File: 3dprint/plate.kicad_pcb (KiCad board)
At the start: 2 copper layers, 129 x 93.3 mm, 49 parts, among them J1 Cutout_TRRS, SW1 SW_PUSH, SW10 SW_PUSH, SW11 SW_PUSH, SW12 SW_PUSH, SW13 SW_PUSH, SW14 SW_PUSH, SW15 SW_PUSH, SW16 SW_PUSH, SW17 SW_PUSH, SW18 SW_PUSH, SW2 SW_PUSH, SW3 SW_PUSH, SW4 SW_PUSH, SW5 SW_PUSH, SW6 SW_PUSH, SW7 SW_PUSH, SW8 SW_PUSH, SW9 SW_PUSH, U1 xiao-ble, U2 xiao-ble

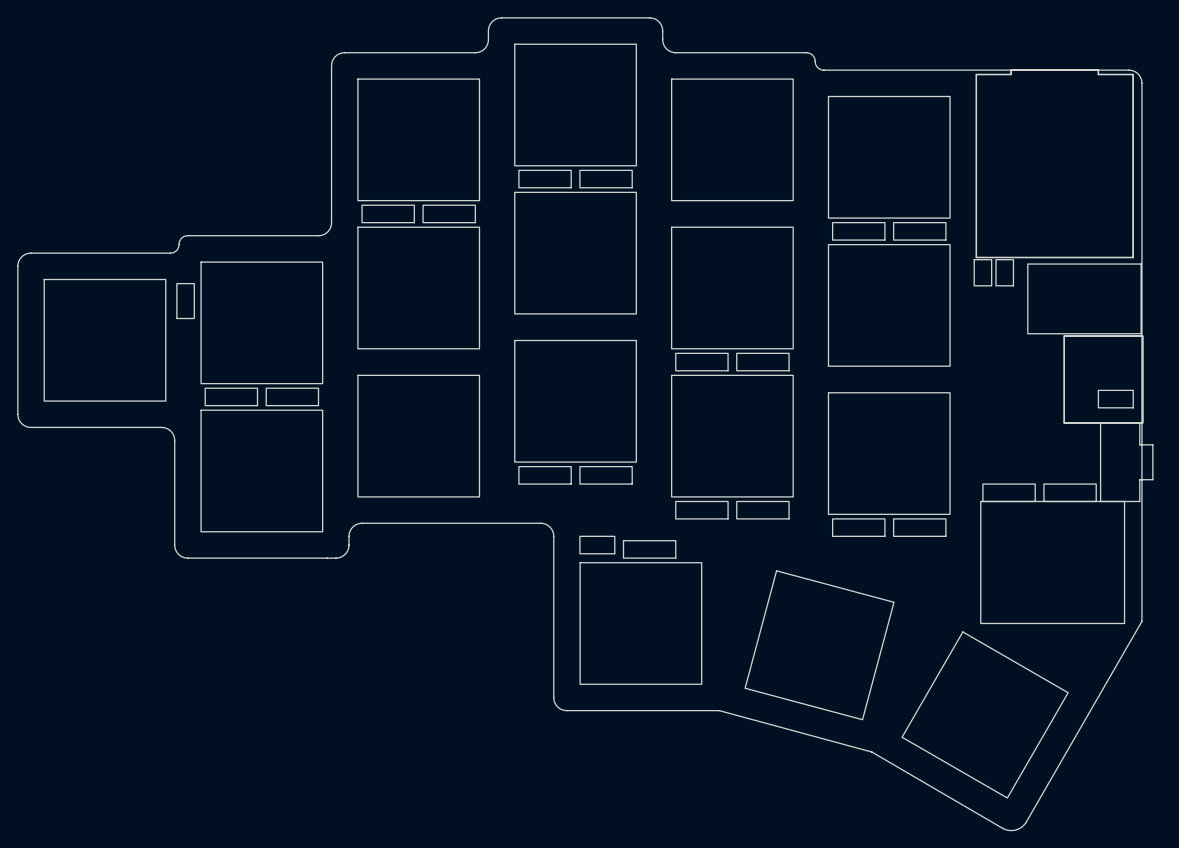
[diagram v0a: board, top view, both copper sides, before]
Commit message: update wired cases
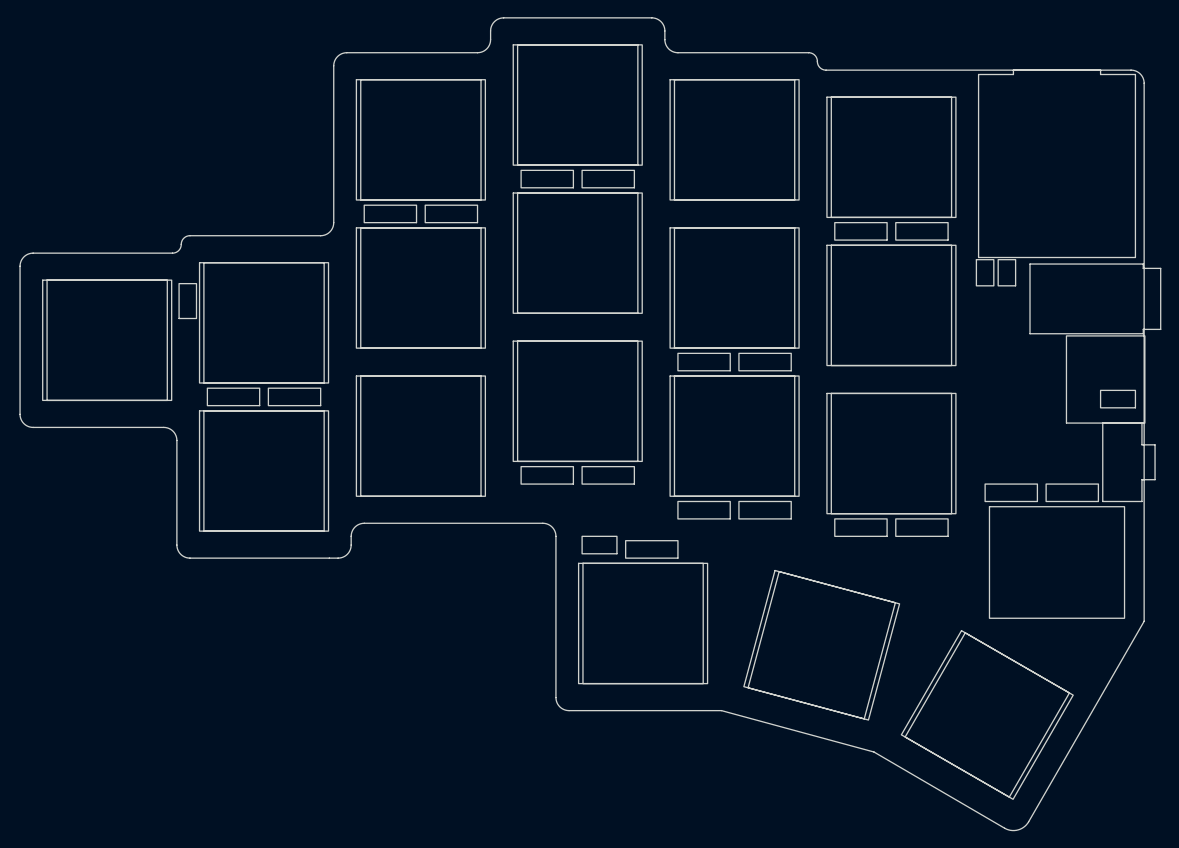
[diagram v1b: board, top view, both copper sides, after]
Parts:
- removed U2: xiao-ble, picachoc:Cutout_xiao
- removed USB2: HRO-TYPE-C-31-M-12, picachoc:Cutout_TypeC
- BATTCONN1, BATTCONN2, BATTCONN3: footprint picachoc:Cutout_JST_PH_S2B-PH-K_1x02_P2.00mm -> zzkeeb:Connector_JST-1x02-2.00mm-cutout
- BATTSW1: footprint picachoc:Cutout_SW_SPDT_PCM12 -> zzkeeb:Switch_SPDT-PCM12-cutout
- D1, D10, D11, D12, D13, D14, D15, D16, D17, D18, D19, D2, D3, D4, D5, D6, D7, D8, D9: footprint picachoc:Cutout_D3_SMD -> zzkeeb:Diode_1N4148-SOD123-cutout
- J1: value Cutout_TRRS -> Cutout_TRRS_resersible; footprint picachoc:Cutout_TRRS -> zzkeeb:Connector_TRRS-cutout-top-resersible
- JP1, JP2: footprint picachoc:Cutout_SolderJumper-2_P1.3mm_Open_TrianglePad1.0x1.5mm -> zzkeeb:SolderJumper-1.3mm-cutout
- RE1: footprint picachoc:Cutout_EC11 -> zzkeeb:RotaryEncoder_EC11-cutout-top-wide
- SW1, SW10, SW11, SW12, SW13, SW14, SW15, SW16, SW17, SW18, SW2, SW3, SW4, SW5, SW6, SW7, SW8, SW9: footprint picachoc:Cutout_ChocV1 -> zzkeeb:Switch_ChocV1-cutout-top
- U1: footprint picachoc:Cutout_xiao -> zzkeeb:MCU_xiao-cutout
- USB1: footprint picachoc:Cutout_TypeC -> zzkeeb:Connector_HRO-TYPE-C-31-M-12-cutout
- moved BATTCONN1 0.25 mm to (135.0, 112.5)
- moved BATTCONN2 0.25 mm to (86.8, 85.5)
- moved BATTCONN3 0.25 mm to (194.5, 95.8)
- moved BATTSW1 0.25 mm to (194.2, 103.0)
- moved D1 0.25 mm to (92.0, 95.5)
- moved D10 0.25 mm to (153.0, 91.5)
- moved D11 0.25 mm to (128.0, 104.5)
- moved D12 0.25 mm to (135.0, 104.5)
- moved D13 0.25 mm to (146.0, 108.5)
- moved D14 0.25 mm to (153.0, 108.5)
- moved D15 0.25 mm to (181.2, 106.5)
- moved D16 0.25 mm to (140.0, 113.0)
- moved D17 0.25 mm to (164.0, 110.5)
- moved D18 0.25 mm to (171.0, 110.5)
- moved D19 0.25 mm to (188.2, 106.5)
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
